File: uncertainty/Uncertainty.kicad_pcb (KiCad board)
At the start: 2 copper layers, 41.9 x 116.8 mm, 49 parts, among them J1 SWITCHCRAFT_35RASMT2AHNTRX, J10 SAMTEC_TSM-103-01-L-SH, J2 SWITCHCRAFT_35RASMT2AHNTRX, J3 SWITCHCRAFT_35RASMT2AHNTRX, J4 SWITCHCRAFT_35RASMT2AHNTRX, J5 SWITCHCRAFT_35RASMT2AHNTRX, J6 SWITCHCRAFT_35RASMT2AHNTRX, J7 SWITCHCRAFT_35RASMT2AHNTRX, J8 SWITCHCRAFT_35RASMT2AHNTRX, J9 SWITCHCRAFT_35RASMT2AHNTRX, U1 VREG_LM1117IMPX-3.3/NOPB, U2 VREG_L7805CDT-TR, U3 MC74ACT05DG, U4 MC74ACT05DG, U5 XIAO-RP2040

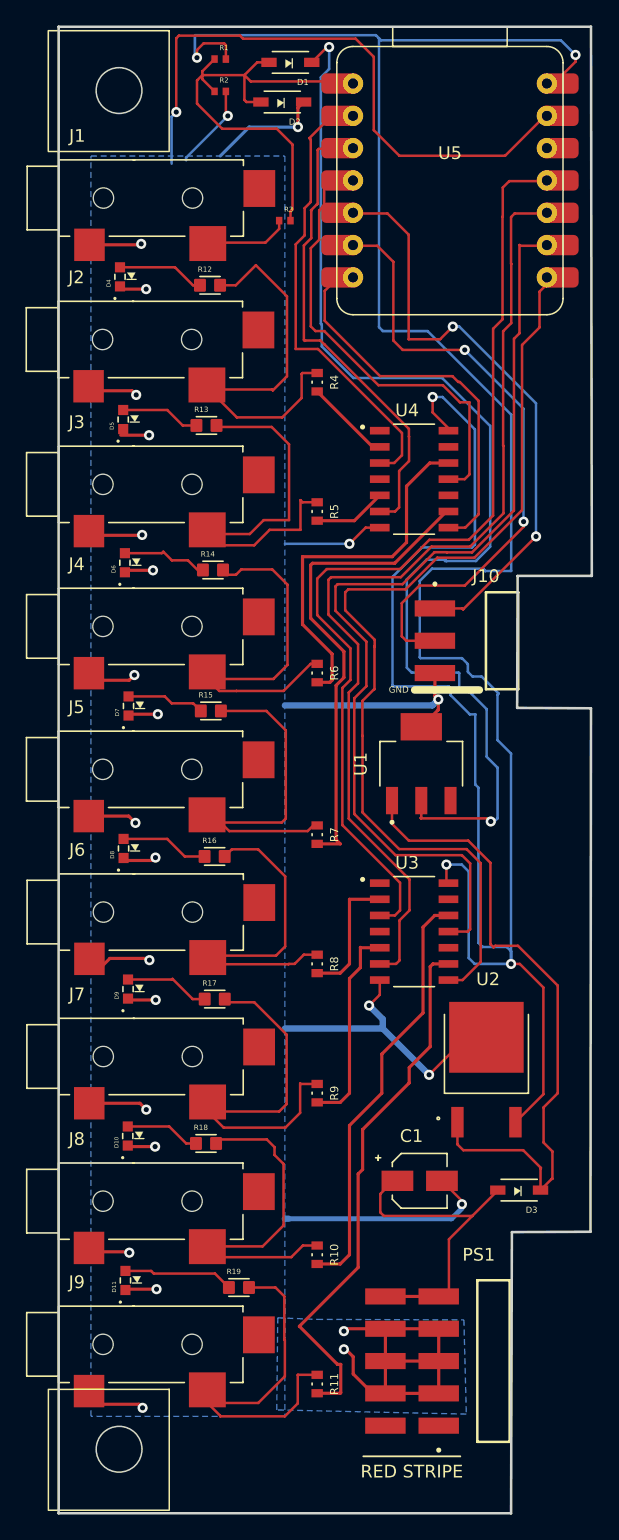
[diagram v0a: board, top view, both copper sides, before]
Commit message: pinout fixes, better nets
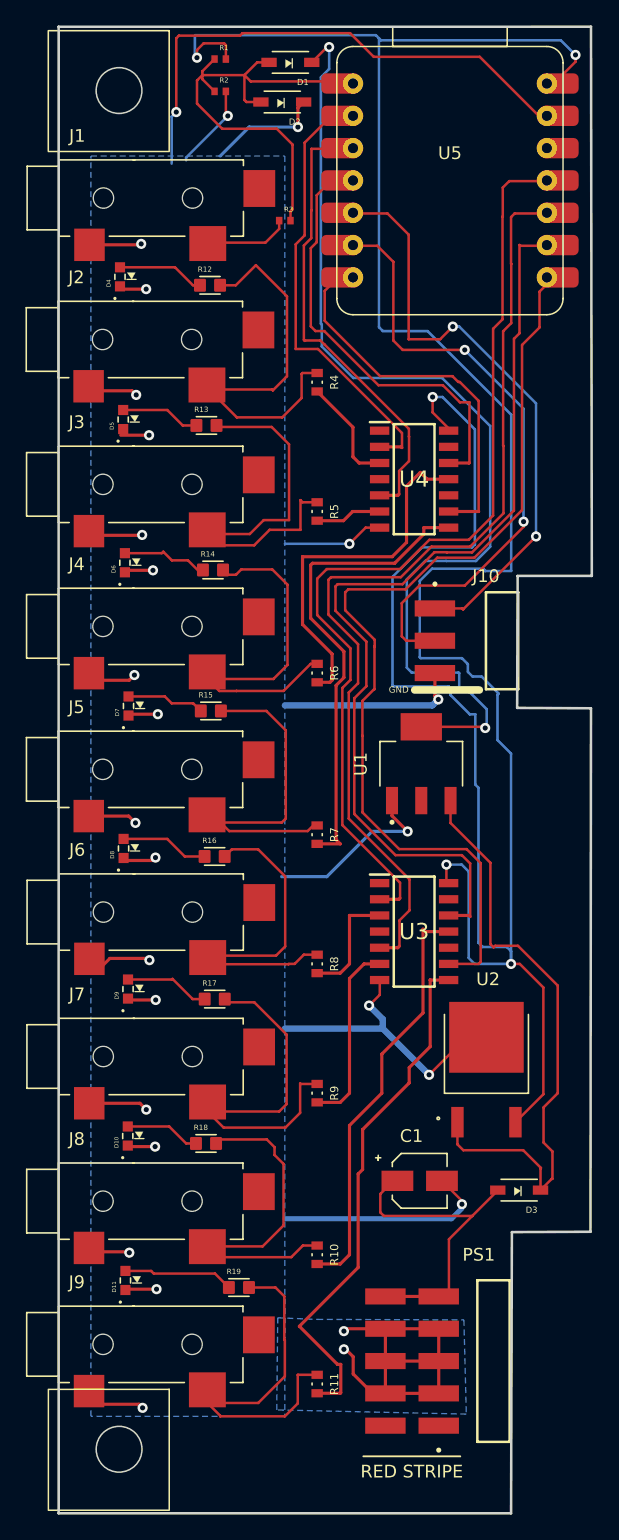
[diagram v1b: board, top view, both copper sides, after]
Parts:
- U3, U4: value MC74ACT05DG -> SN74HCS125QBQARQ1; footprint Import Library:MC74ACT05DG -> Import Library:SN74HCS125QBQARQ1
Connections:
- D1 pad A: (no net) -> Signal-In
- D1 pad C: Power -> 3.3V
- D10 pad A: (no net) -> Signal-Out7
- D11 pad A: (no net) -> Signal-Out8
- D2 pad A: (no net) -> Signal-In
- D4 pad A: (no net) -> Signal-Out1
- D5 pad A: (no net) -> Signal-Out2
- D6 pad A: (no net) -> Signal-Out3
- D7 pad A: (no net) -> Signal-Out4
- D8 pad A: (no net) -> Signal-Out5
- D9 pad A: (no net) -> Signal-Out6
- J1 pad 4: (no net) -> Signal-In
- J10 pad 01: (no net) -> i2c-SDA
- J10 pad 02: (no net) -> i2c-SCL
- J2 pad 4: (no net) -> Signal-Out1
- J3 pad 4: (no net) -> Signal-Out2
- J4 pad 4: (no net) -> Signal-Out3
- J5 pad 4: (no net) -> Signal-Out4
- J6 pad 4: (no net) -> Signal-Out5
- J7 pad 4: (no net) -> Signal-Out6
- J8 pad 4: (no net) -> Signal-Out7
- J9 pad 4: (no net) -> Signal-Out8
- R1 pad 1: (no net) -> Signal-In
- R1 pad 2: Power -> 5V
- R10 pad 1: (no net) -> Signal-Out7
- R10 pad 2: (no net) -> Signal-Out7
- R11 pad 1: (no net) -> Signal-Out8
- R11 pad 2: (no net) -> Signal-Out8
- R12 pad 1: (no net) -> Signal-Out1
- R12 pad 2: (no net) -> Signal-Out1
- R13 pad 1: (no net) -> Signal-Out2
- R13 pad 2: (no net) -> Signal-Out2
- R14 pad 1: (no net) -> Signal-Out3
- R14 pad 2: (no net) -> Signal-Out3
- R15 pad 1: (no net) -> Signal-Out4
- R15 pad 2: (no net) -> Signal-Out4
- R16 pad 1: (no net) -> Signal-Out5
- R16 pad 2: (no net) -> Signal-Out5
- R17 pad 1: (no net) -> Signal-Out6
- R17 pad 2: (no net) -> Signal-Out6
- R18 pad 1: (no net) -> Signal-Out7
- R18 pad 2: (no net) -> Signal-Out7
- R19 pad 2: (no net) -> Signal-Out8
- R2 pad 1: (no net) -> Signal-In
- R3 pad 1: (no net) -> Signal-In
- R3 pad 2: (no net) -> Signal-In
- R4 pad 1: (no net) -> Signal-Out1
- R4 pad 2: (no net) -> Signal-Out1
- R5 pad 1: (no net) -> Signal-Out2
- R5 pad 2: (no net) -> Signal-Out2
- R6 pad 1: (no net) -> Signal-Out3
- R6 pad 2: (no net) -> Signal-Out3
- R7 pad 1: (no net) -> Signal-Out4
- R7 pad 2: (no net) -> Signal-Out4
- R8 pad 1: (no net) -> Signal-Out5
- R8 pad 2: (no net) -> Signal-Out5
- R9 pad 1: (no net) -> Signal-Out6
- R9 pad 2: (no net) -> Signal-Out6
- U1 pad 1: Power -> Ground
- U1 pad 3: (no net) -> Power
- U1 pad 4: Ground -> 3.3V
- U2 pad 2: Power -> 5V
- U3 pad 11: (no net) -> Signal-Out7
- U3 pad 12: (no net) -> Signal-Out7
- U3 pad 14: Power -> 5V
- U3 pad 2: (no net) -> Signal-Out5
- U3 pad 3: (no net) -> Signal-Out5
- U3 pad 5: (no net) -> Signal-Out6
- U3 pad 6: (no net) -> Signal-Out6
- U3 pad 8: (no net) -> Signal-Out8
- U3 pad 9: (no net) -> Signal-Out8
- U4 pad 11: (no net) -> Signal-Out3
- U4 pad 12: (no net) -> Signal-Out3
- U4 pad 14: Power -> 5V
- U4 pad 2: (no net) -> Signal-Out1
- U4 pad 3: (no net) -> Signal-Out1
- U4 pad 5: (no net) -> Signal-Out2
- U4 pad 6: (no net) -> Signal-Out2
- U4 pad 8: (no net) -> Signal-Out4
- U4 pad 9: (no net) -> Signal-Out4
- U5 pad 1: (no net) -> Signal-In
- U5 pad 10: (no net) -> Signal-Out6
- U5 pad 11: (no net) -> Signal-Out5
- U5 pad 14: Power -> 5V
- U5 pad 2: (no net) -> Signal-Out1
- U5 pad 3: (no net) -> Signal-Out2
- U5 pad 4: (no net) -> Signal-Out3
- U5 pad 5: (no net) -> i2c-SDA
- U5 pad 6: (no net) -> i2c-SCL
- U5 pad 7: (no net) -> Signal-Out4
- U5 pad 8: (no net) -> Signal-Out8
- U5 pad 9: (no net) -> Signal-Out7
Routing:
- net (no net): track 1063.4 -> 0.00 mm, vias 13 -> 0
- net Power: track 391.4 -> 72.2 mm, vias 2 -> 0
- net 5V: track 0.00 -> 222.1 mm, vias 0 -> 5
- net Signal-Out8: track 0.00 -> 154.0 mm
- net Signal-Out7: track 0.00 -> 144.5 mm
- net Signal-Out6: track 0.00 -> 128.2 mm
- net Signal-Out5: track 0.00 -> 120.8 mm
- net Signal-Out4: track 0.00 -> 102.0 mm
- net Signal-Out3: track 0.00 -> 101.6 mm
- net Signal-Out1: track 0.00 -> 82.9 mm
- net 3.3V: track 0.00 -> 80.5 mm, vias 0 -> 2
- net Signal-Out2: track 0.00 -> 78.8 mm
- net i2c-SCL: track 0.00 -> 49.5 mm, vias 0 -> 2
- net i2c-SDA: track 0.00 -> 47.5 mm, vias 0 -> 2
- net Signal-In: track 0.00 -> 44.8 mm
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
